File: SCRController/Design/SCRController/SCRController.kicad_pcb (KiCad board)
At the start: 2 copper layers, 100 x 100 mm, 42 parts, among them J1 VALT, J2 SAL_TRIAC, Q1 2N2907A, Q2 2N2222A, Q3 2N2222A, Q4 2N2907A, U1 TL084, U2 TL084, U3 LM7815_TO220, U4 LM7915_TO220, U5 MOC3011M

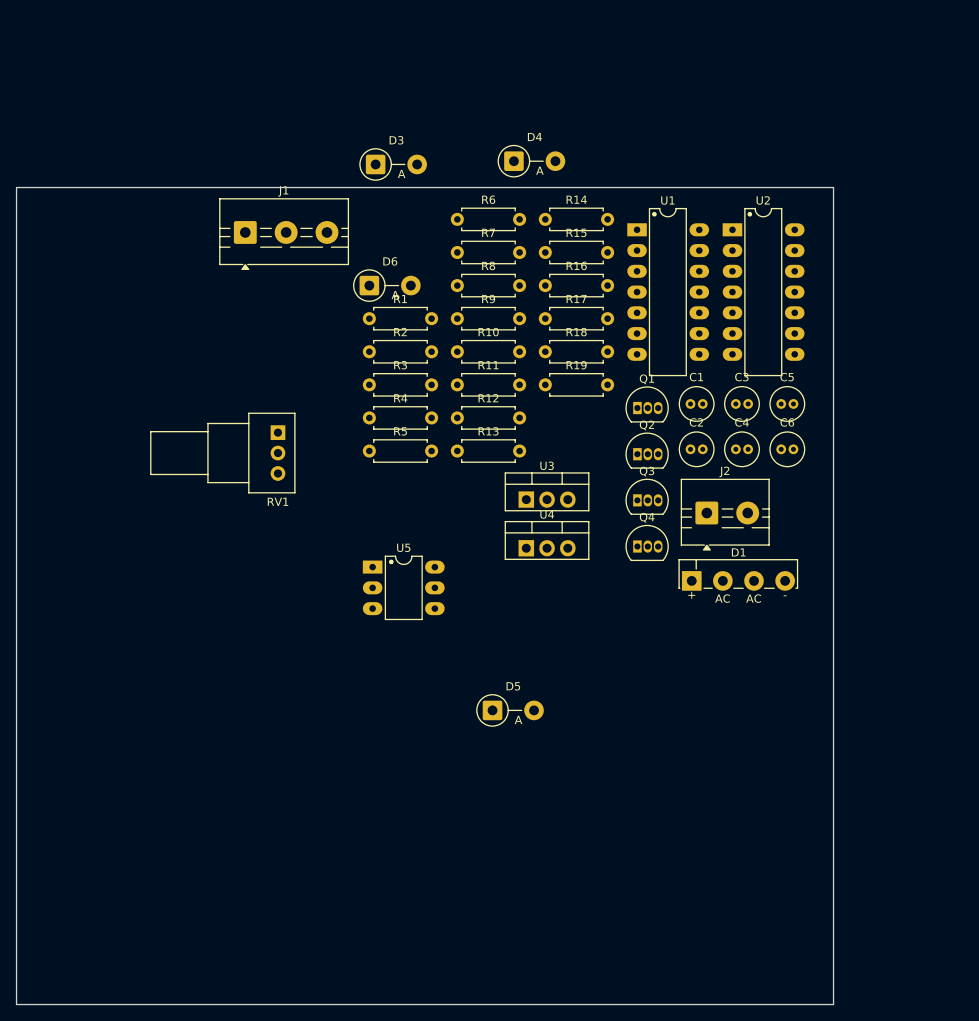
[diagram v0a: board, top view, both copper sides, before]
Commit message: Placed Footprints and first routed
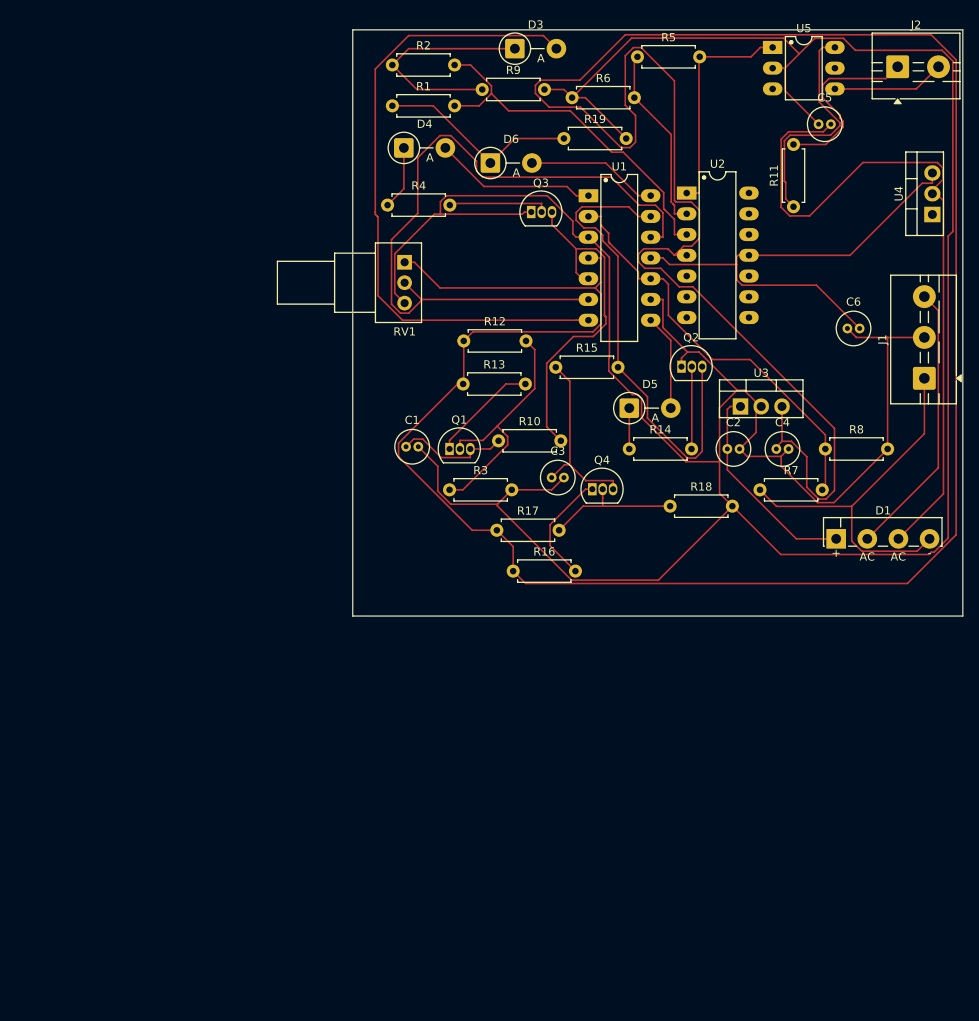
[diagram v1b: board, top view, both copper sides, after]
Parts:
- moved J1 85.0 mm to (161.1, 86.3), turned to 90 degrees
- moved U5 80.3 mm to (142.6, 45.9)
- moved U4 64.3 mm to (162.1, 66.3), turned to 90 degrees
- moved J2 59.4 mm to (157.8, 48.2)
- moved R5 58.4 mm to (126.0, 47.0)
- moved R8 49.3 mm to (149.0, 95.0)
- moved R7 47.1 mm to (141.0, 100.0)
- moved R11 46.6 mm to (145.1, 65.3), turned to 90 degrees
- moved D5 40.6 mm to (125.0, 90.0)
- moved Q3 37.6 mm to (113.0, 66.0)
- moved R2 35.2 mm to (96.0, 48.0)
- moved C1 35.2 mm to (97.7, 94.7)
- moved R16 35.2 mm to (110.8, 110.0)
- moved C5 34.5 mm to (148.2, 55.2)
- moved R19 30.2 mm to (117.0, 57.0)
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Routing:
- net DERCENT: track 0.00 -> 405.7 mm
- net VCC: track 0.00 -> 388.7 mm
- net VDC-: track 0.00 -> 87.7 mm
- net VCOMP: track 0.00 -> 87.7 mm
- net Net-(D3-A): track 0.00 -> 79.6 mm
- net VEE: track 0.00 -> 60.1 mm
- net Net-(Q2-C): track 0.00 -> 58.9 mm
- net VSync: track 0.00 -> 51.4 mm
- net VA+: track 0.00 -> 46.3 mm
- net Net-(U2A-+): track 0.00 -> 45.2 mm
- net Net-(Q3-C): track 0.00 -> 42.3 mm
- net VA-: track 0.00 -> 34.0 mm
- net Net-(Q1-B): track 0.00 -> 31.3 mm
- net Net-(R11-Pad1): track 0.00 -> 28.6 mm
- net A1: track 0.00 -> 28.1 mm
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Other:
- board size 100 x 100 mm -> 74.7 x 71.8 mm
